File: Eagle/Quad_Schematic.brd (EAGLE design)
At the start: 47 x 28 mm, 36 parts, among them J1 FTDI_DEVICE, M1 WIRELESS-NRF24L01, U1 ATMEGA328P_TQFP, U2 GY-521MPU6050

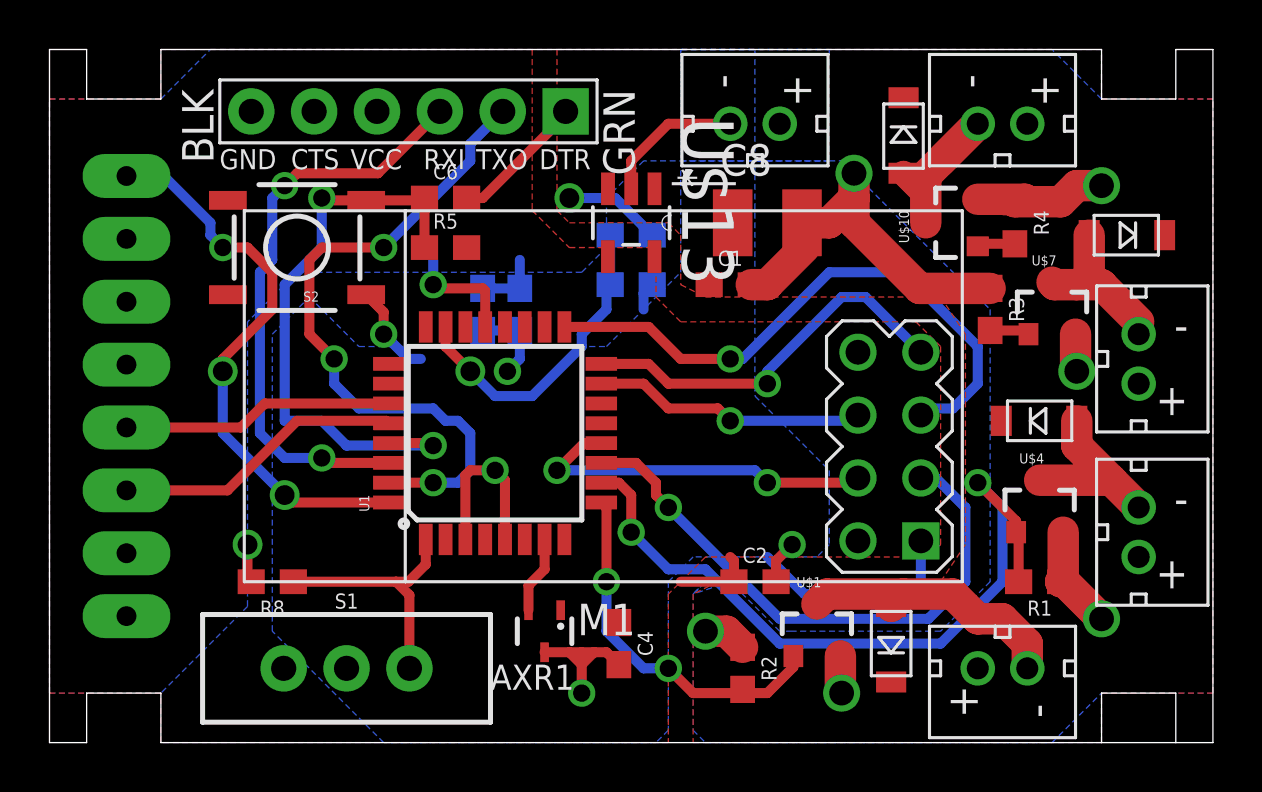
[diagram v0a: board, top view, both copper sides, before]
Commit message: jeffrey approved this
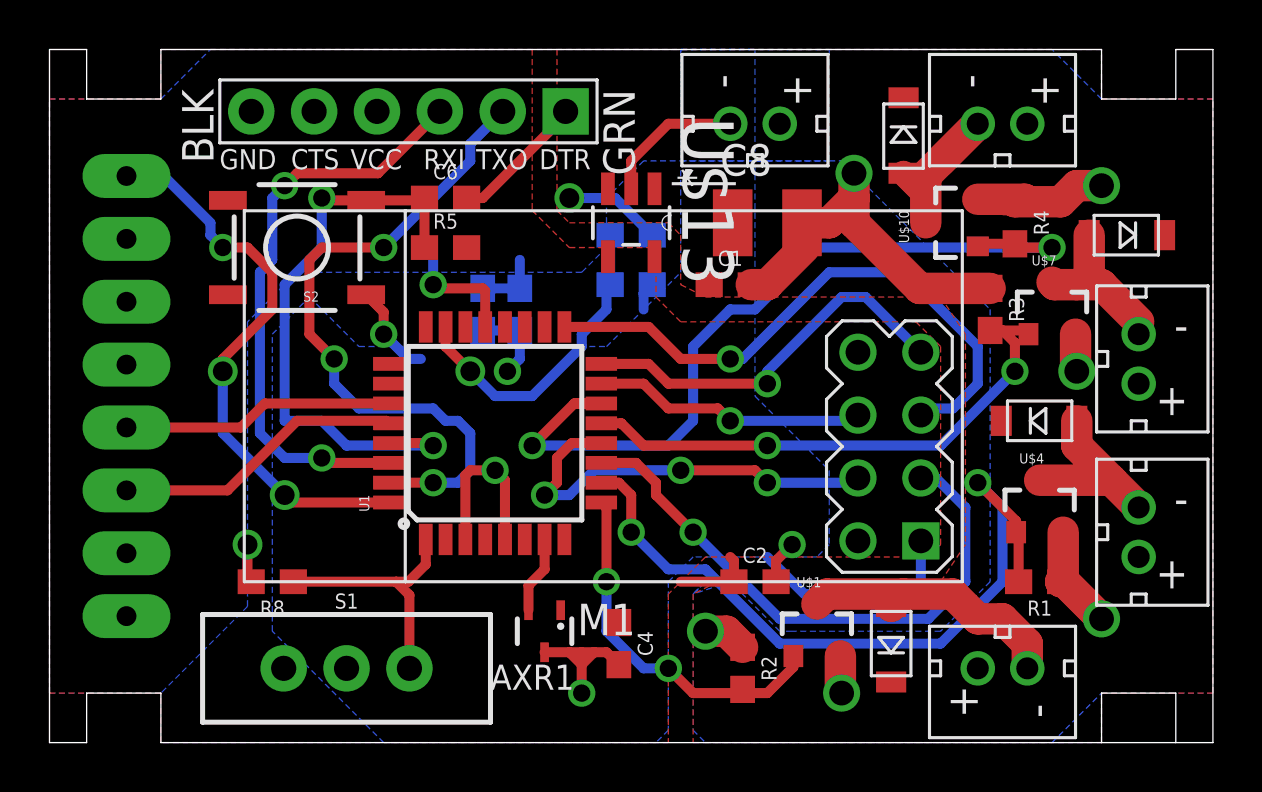
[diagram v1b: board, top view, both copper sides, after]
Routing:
- net M4: track 1.54 -> 33.8 mm, vias 0 -> 2
- net M3: track 1.61 -> 21.8 mm, vias 0 -> 2
- net CS: track 15.1 -> 17.8 mm, vias 2 -> 3
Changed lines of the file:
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@@
 <layer number="25" name="tNames" color="7" fill="1" visible="yes" active="yes"/>
 <layer number="26" name="bNames" color="7" fill="1" visible="yes" active="yes"/>
-<layer number="27" name="tValues" color="7" fill="1" visible="yes" active="yes"/>
-<layer number="28" name="bValues" color="7" fill="1" visible="yes" active="yes"/>
+<layer number="27" name="tValues" color="7" fill="1" visible="no" active="yes"/>
+<layer number="28" name="bValues" color="7" fill="1" visible="no" active="yes"/>
 <layer number="29" name="tStop" color="7" fill="3" visible="no" active="yes"/>
 <layer number="30" name="bStop" color="7" fill="6" visible="no" active="yes"/>
@@
 <layer number="35" name="tGlue" color="7" fill="4" visible="no" active="yes"/>
 <layer number="36" name="bGlue" color="7" fill="5" visible="no" active="yes"/>
-<layer number="37" name="tTest" color="7" fill="1" visible="yes" active="yes"/>
-<layer number="38" name="bTest" color="7" fill="1" visible="yes" active="yes"/>
+<layer number="37" name="tTest" color="7" fill="1" visible="no" active="yes"/>
+<layer number="38" name="bTest" color="7" fill="1" visible="no" active="yes"/>
 <layer number="39" name="tKeepout" color="4" fill="11" visible="yes" active="yes"/>
 <layer number="40" name="bKeepout" color="1" fill="11" visible="yes" active="yes"/>
@@
 <layer number="42" name="bRestrict" color="1" fill="10" visible="yes" active="yes"/>
 <layer number="43" name="vRestrict" color="2" fill="10" visible="yes" active="yes"/>
-<layer number="44" name="Drills" color="7" fill="1" visible="yes" active="yes"/>
+<layer number="44" name="Drills" color="7" fill="1" visible="no" active="yes"/>
 <layer number="45" name="Holes" color="7" fill="1" visible="yes" active="yes"/>
 <layer number="46" name="Milling" color="3" fill="1" visible="yes" active="yes"/>
@@
 <wire x1="23.7" y1="11.3" x2="24.5" y2="10.5" width="0.4064" layer="1"/>
 <wire x1="24.5" y1="10.5" x2="24.5" y2="10" width="0.4064" layer="1"/>
-<wire x1="24.5" y1="10" x2="25" y2="9.5" width="0.4064" layer="1"/>
-<via x="25" y="9.5" extent="1-16" drill="0.7"/>
-<wire x1="25" y1="9.5" x2="29.5" y2="5" width="0.4064" layer="16"/>
+<wire x1="24.5" y1="10" x2="26" y2="8.5" width="0.4064" layer="1"/>
+<via x="26" y="8.5" extent="1-16" drill="0.7"/>
+<wire x1="26" y1="8.5" x2="29.5" y2="5" width="0.4064" layer="16"/>
 <wire x1="29.5" y1="5" x2="35.5" y2="5" width="0.4064" layer="16"/>
 </signal>
@@
 <contactref element="M1" pad="4"/>
 <contactref element="U1" pad="12"/>
-<wire x1="32.66" y1="10.69" x2="32.35" y2="11" width="0.4064" layer="16"/>
-<wire x1="22.2926" y1="12.1" x2="21.6" y2="12.1" width="0.4064" layer="1"/>
-<wire x1="21.6" y1="12.1" x2="20.5" y2="11" width="0.4064" layer="1"/>
-<via x="20.5" y="11" extent="1-16" drill="0.7"/>
-<wire x1="20.5" y1="11" x2="28.5" y2="11" width="0.4064" layer="16"/>
-<wire x1="28.5" y1="11" x2="29" y2="10.5" width="0.4064" layer="16"/>
+<wire x1="21.6" y1="12.1" x2="22.2926" y2="12.1" width="0.4064" layer="1"/>
+<via x="25.5" y="11" extent="1-16" drill="0.7"/>
+<wire x1="25.5" y1="11" x2="28.5" y2="11" width="0.4064" layer="1"/>
+<wire x1="28.5" y1="11" x2="29" y2="10.5" width="0.4064" layer="1"/>
 <via x="29" y="10.5" extent="1-16" drill="0.7"/>
-<wire x1="29" y1="10.5" x2="32.47" y2="10.5" width="0.4064" layer="1"/>
-<wire x1="32.47" y1="10.5" x2="32.66" y2="10.69" width="0.4064" layer="1"/>
+<wire x1="29" y1="10.5" x2="32.47" y2="10.5" width="0.4064" layer="16"/>
+<wire x1="32.47" y1="10.5" x2="32.66" y2="10.69" width="0.4064" layer="16"/>
+<wire x1="22.2926" y1="12.1" x2="21.1" y2="12.1" width="0.4064" layer="1"/>
+<wire x1="21.1" y1="12.1" x2="20.5" y2="11.5" width="0.4064" layer="1"/>
+<wire x1="20.5" y1="11.5" x2="20.5" y2="10.5" width="0.4064" layer="1"/>
+<wire x1="20.5" y1="10.5" x2="20" y2="10" width="0.4064" layer="1"/>
+<via x="20" y="10" extent="1-16" drill="0.7"/>
+<wire x1="20" y1="10" x2="21" y2="10" width="0.4064" layer="16"/>
+<wire x1="21" y1="10" x2="22" y2="11" width="0.4064" layer="16"/>
+<wire x1="22" y1="11" x2="25.5" y2="11" width="0.4064" layer="16"/>
 </signal>
 <signal name="M4">
@@
 <wire x1="39" y1="20.15" x2="37.6" y2="20.15" width="0.4064" layer="1"/>
 <wire x1="37.6" y1="20.15" x2="37.5" y2="20.05" width="0.4064" layer="1"/>
-<wire x1="22.2926" y1="13.7" x2="37.5" y2="20.05" width="0" layer="19" extent="1-1"/>
+<wire x1="21.2" y1="13.7" x2="22.2926" y2="13.7" width="0.4064" layer="1"/>
+<wire x1="26" y1="13" x2="26" y2="16" width="0.4064" layer="16"/>
+<wire x1="26" y1="16" x2="27.5" y2="17.5" width="0.4064" layer="16"/>
+<wire x1="27.5" y1="17.5" x2="28.5" y2="17.5" width="0.4064" layer="16"/>
+<wire x1="28.5" y1="17.5" x2="31" y2="20" width="0.4064" layer="16"/>
+<wire x1="31" y1="20" x2="40.5" y2="20" width="0.4064" layer="16"/>
+<via x="40.5" y="20" extent="1-16" drill="0.7"/>
+<wire x1="40.5" y1="20" x2="39.15" y2="20" width="0.4064" layer="1"/>
+<wire x1="39.15" y1="20" x2="39" y2="20.15" width="0.4064" layer="1"/>
+<wire x1="22.2926" y1="13.7" x2="21.2" y2="13.7" width="0.4064" layer="1"/>
+<via x="19.5" y="12" extent="1-16" drill="0.7"/>
+<wire x1="19.5" y1="12" x2="25" y2="12" width="0.4064" layer="16"/>
+<wire x1="21.2" y1="13.7" x2="19.5" y2="12" width="0.4064" layer="1"/>
+<wire x1="25" y1="12" x2="26" y2="13" width="0.4064" layer="16"/>
 </signal>
 <signal name="OSC1">
@@
 <contactref element="R3" pad="2"/>
 <contactref element="U$7" pad="1"/>
-<wire x1="38" y1="16.65" x2="39.4" y2="16.65" width="0.4064" layer="1"/>
+<wire x1="38.5" y1="16.65" x2="38" y2="16.65" width="0.4064" layer="1"/>
+<wire x1="38.5" y1="16.65" x2="39.4" y2="16.65" width="0.4064" layer="1"/>
 <wire x1="39.55" y1="16.5" x2="39.4" y2="16.65" width="0.4064" layer="1"/>
-<wire x1="22.2926" y1="12.9" x2="38" y2="16.65" width="0" layer="19" extent="1-1"/>
+<via x="29" y="12" extent="1-16" drill="0.7"/>
+<wire x1="29" y1="12" x2="36" y2="12" width="0.4064" layer="16"/>
+<wire x1="36" y1="12" x2="39" y2="15" width="0.4064" layer="16"/>
+<via x="39" y="15" extent="1-16" drill="0.7"/>
+<wire x1="39" y1="15" x2="39" y2="16.15" width="0.4064" layer="1"/>
+<wire x1="39" y1="16.15" x2="38.5" y2="16.65" width="0.4064" layer="1"/>
+<wire x1="22.2926" y1="12.9" x2="23.1" y2="12.9" width="0.4064" layer="1"/>
+<wire x1="23.1" y1="12.9" x2="24" y2="12" width="0.4064" layer="1"/>
+<wire x1="24" y1="12" x2="29" y2="12" width="0.4064" layer="1"/>
 </signal>
 <signal name="MOSI">

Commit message: GOGOGO
basically done?
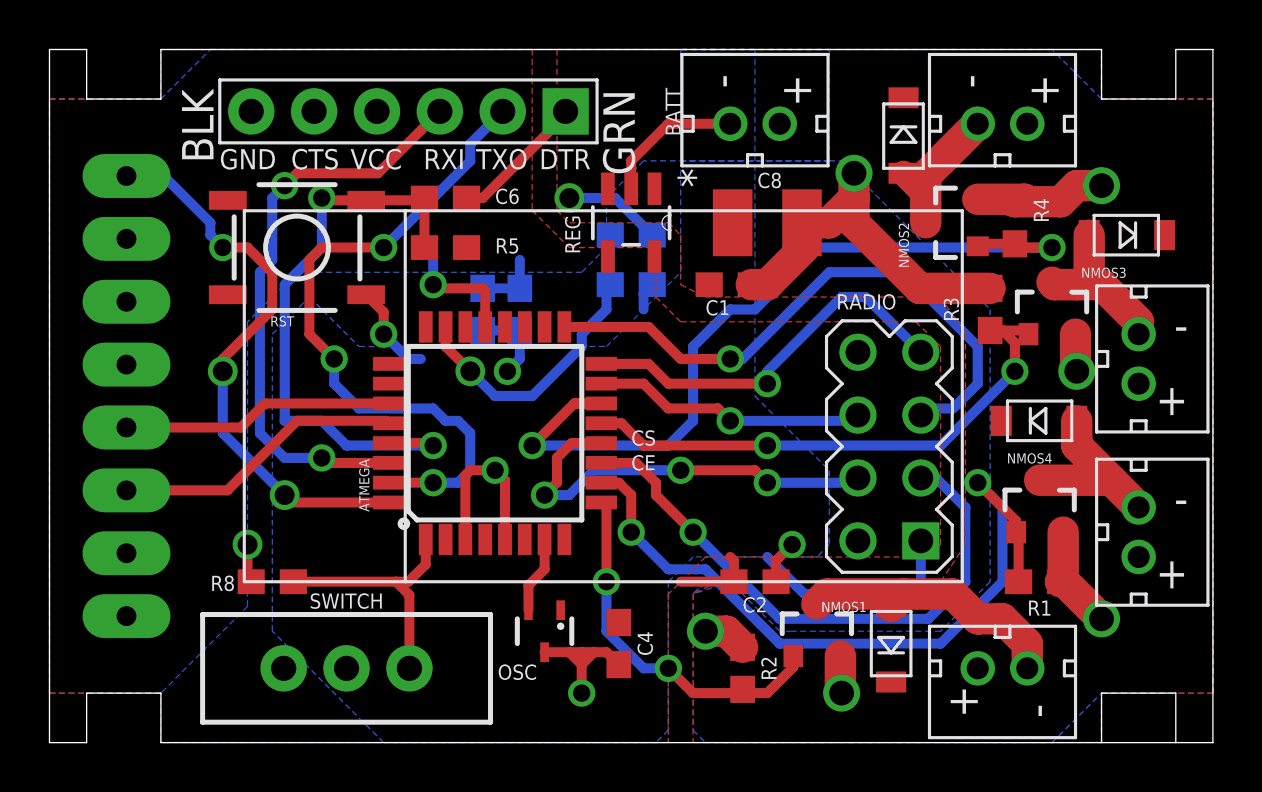
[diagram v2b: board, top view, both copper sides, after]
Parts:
- renumbered AXR1 to OSC, M1 to RADIO, S1 to SWITCH, S2 to RST, U$1 to NMOS1, U$10 to NMOS2, U$13 to REG, U$4 to NMOS4, U$7 to NMOS3, U1 to ATMEGA
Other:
- board text added: "BATT"
- board text added: "CE"
- board text added: "CS"
- board text added: "Team Lucky 7"
